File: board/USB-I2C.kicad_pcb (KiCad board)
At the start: 2 copper layers, 55 x 18 mm, 16 parts, among them J1 USB_OTG, J2 Conn_01x06, J3 Conn_01x06, U1 SPX3819, U2 ATSAMD11C14A-SS, X1 I2C-6P, X2 I2C, X3 SWD

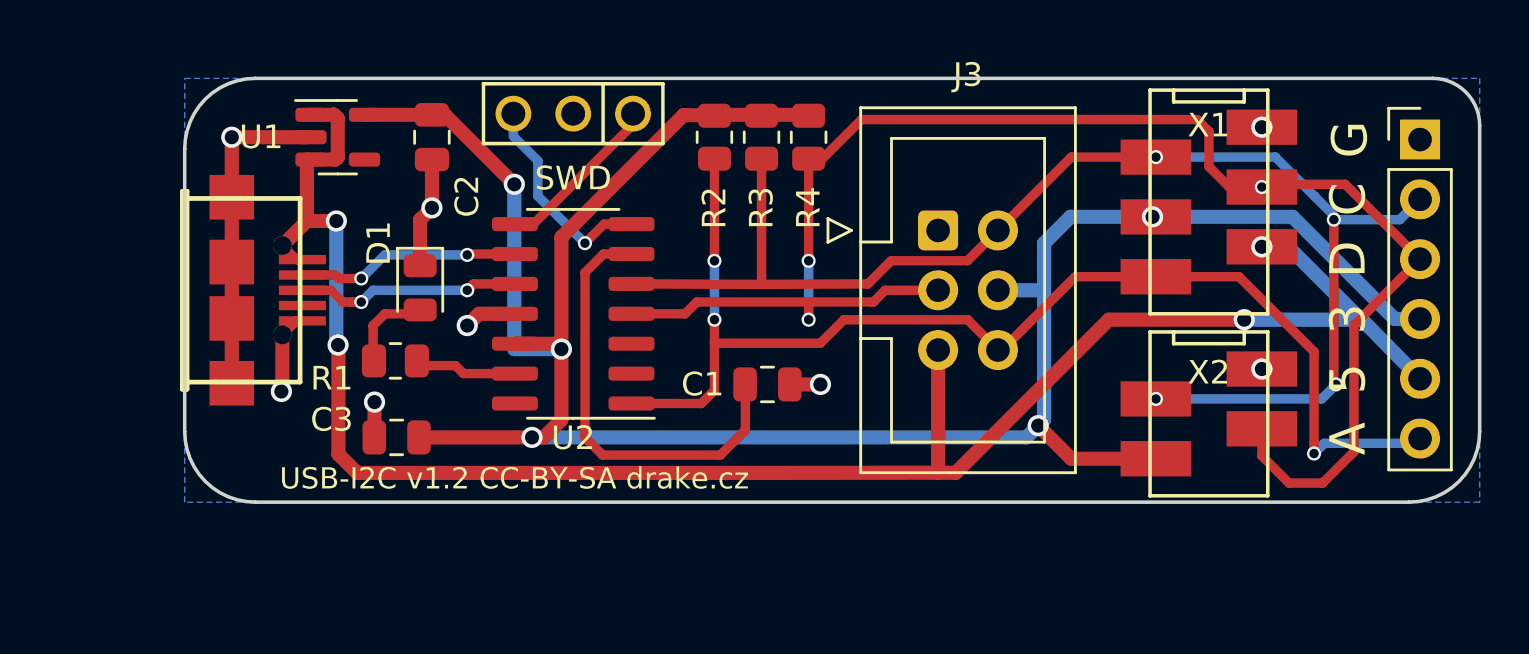
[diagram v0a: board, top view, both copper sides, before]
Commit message: WIP
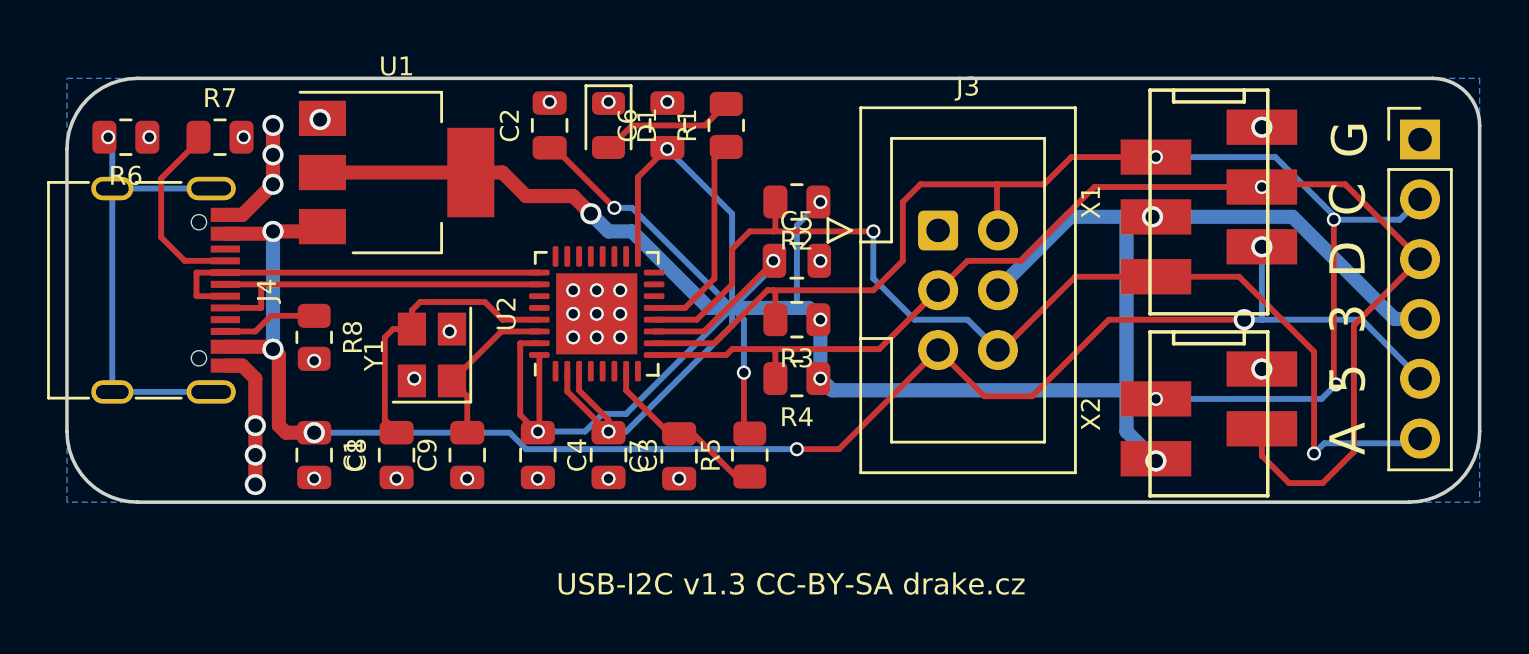
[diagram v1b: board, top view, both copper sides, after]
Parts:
- removed the C3 at (156.0, 114.2)
- removed the J1 at (149.0, 108.0)
- removed X3: SWD, Drake:SWD
- added C1: 10u, Capacitor_SMD:C_0805_2012Metric, F.Cu at (152.5, 115.0)
- added C4: 100n, Capacitor_SMD:C_0805_2012Metric, F.Cu at (162.0, 115.0)
- added C5: 100n, Capacitor_SMD:C_0805_2012Metric, F.Cu at (173.0, 106.8)
- added C6: 100n, Capacitor_SMD:C_0805_2012Metric, F.Cu at (167.5, 101.0)
- added C7: 1u, Capacitor_SMD:C_0805_2012Metric, F.Cu at (168.0, 115.0)
- added C8: 15p, Capacitor_SMD:C_0805_2012Metric, F.Cu at (156.0, 115.0)
- added C9: 15p, Capacitor_SMD:C_0805_2012Metric, F.Cu at (159.0, 115.0)
- added J4: USB_C_Receptacle, Connector_USB:USB_C_Receptacle_G-Switch_GT-USB-7010ASV, F.Cu at (145.0, 108.0)
- added R5: 10k, Resistor_SMD:R_0805_2012Metric, F.Cu at (171.0, 115.0)
- added R6: 1M, Resistor_SMD:R_0805_2012Metric, F.Cu at (144.5, 101.5)
- added R7: 5.11k 1%, Resistor_SMD:R_0805_2012Metric, F.Cu at (148.5, 101.5)
- added R8: 5.11k 1%, Resistor_SMD:R_0805_2012Metric, F.Cu at (152.5, 110.0)
- added Y1: 40MHz, Crystal:Crystal_SMD_3225-4Pin_3.2x2.5mm, F.Cu at (157.5, 110.8)
- C2: value 1u -> 10u
- U1: value SPX3819 -> LM1117MP-3.3; footprint Package_TO_SOT_SMD:SOT-23-5 -> Package_TO_SOT_SMD:SOT-223-3_TabPin2
- U2: value ATSAMD11C14A-SS -> ESP32-C3; footprint Package_SO:SOIC-14_3.9x8.7mm_P1.27mm -> Package_DFN_QFN:QFN-32-1EP_5x5mm_P0.5mm_EP3.45x3.45mm
- moved R1 17.2 mm to (170.0, 101.0), turned to 90 degrees
- moved D1 10.6 mm to (165.0, 101.0)
- moved R4 10.3 mm to (173.0, 111.8), turned to 180 degrees
- moved R3 7.89 mm to (173.0, 109.2), turned to 180 degrees
- moved C3 7.39 mm to (165.0, 115.0), turned to -90 degrees
- moved C2 5.02 mm to (162.5, 101.0), turned to 90 degrees
- moved R2 4.45 mm to (173.0, 104.2), turned to 180 degrees
- moved U1 2.92 mm to (156.0, 103.0)
- moved U2 1.00 mm to (164.5, 109.0), turned to 90 degrees
- renumbered C1 to C3, J2 to J1
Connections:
- C3 pad 1: Net-(C1-Pad1) -> +3V3
- U1 pad 1: +5V -> GND
- U1 pad 2: GND -> +3V3
- U2 pad 1: /ALERT -> unconnected-(U2-LNA_IN-Pad1)
- U2 pad 10: /USB_DP -> /SCL
- U2 pad 11: GND -> +3V3
- U2 pad 12: +3V3 -> /ALERT
- U2 pad 2: unconnected-(U2-Pad2) -> +3V3
- U2 pad 3: unconnected-(U2-Pad3) -> +3V3
- U2 pad 4: /SDA -> unconnected-(U2-XTAL_32K_P/ADC1_CH0-Pad4)
- U2 pad 5: /SCL -> unconnected-(U2-XTAL_32K_N/ADC1_CH1-Pad5)
- U2 pad 6: Net-(C1-Pad1) -> unconnected-(U2-GPIO2/ADC1_CH2-Pad6)
- U2 pad 7: /SWCLK -> Net-(U2-CHIP_EN)
- U2 pad 8: /SWDIO -> unconnected-(U2-GPIO3/ADC1_CH3-Pad8)
- U2 pad 9: /USB_DM -> /SDA
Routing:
- net +3V3: track 100.8 -> 149.0 mm, vias 5 -> 12
- net Net-(J4-SHIELD): track 0.00 -> 19.3 mm, vias 0 -> 1
- net Net-(C1-Pad1): track 18.8 -> 0.00 mm
- net GND: track 26.7 -> 11.1 mm, vias 8 -> 33
- net /SDA: track 66.5 -> 53.6 mm, vias 3 -> 1
- net Net-(U2-XTAL_N): track 0.00 -> 12.2 mm
- net +5V: track 81.5 -> 71.6 mm, vias 4 -> 6
- net /SWCLK: track 9.41 -> 0.00 mm, vias 1 -> 0
- net Net-(J4-CC1): track 0.00 -> 8.05 mm
- net Net-(U2-CHIP_EN): track 0.00 -> 7.58 mm
- net /USB_DM: track 9.52 -> 16.8 mm, vias 2 -> 0
- net /SWDIO: track 7.23 -> 0.00 mm
- net Net-(U2-XTAL_P): track 0.00 -> 7.05 mm
- net /USB_DP: track 9.55 -> 15.9 mm, vias 2 -> 0
- net /ALERT: track 52.4 -> 47.4 mm, vias 3 -> 2
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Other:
- board size 55 x 18 mm -> 60 x 18 mm
- rule pad_to_mask_clearance: 0.2 -> 0.05
- rule solder_mask_min_width: 0.25 -> 0.254
- board text added: "USB-I2C v1.3 CC-BY-SA drake.cz"
- board text removed: "SWD"
- board text removed: "USB-I2C v1.2 CC-BY-SA drake.cz"

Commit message: WIP
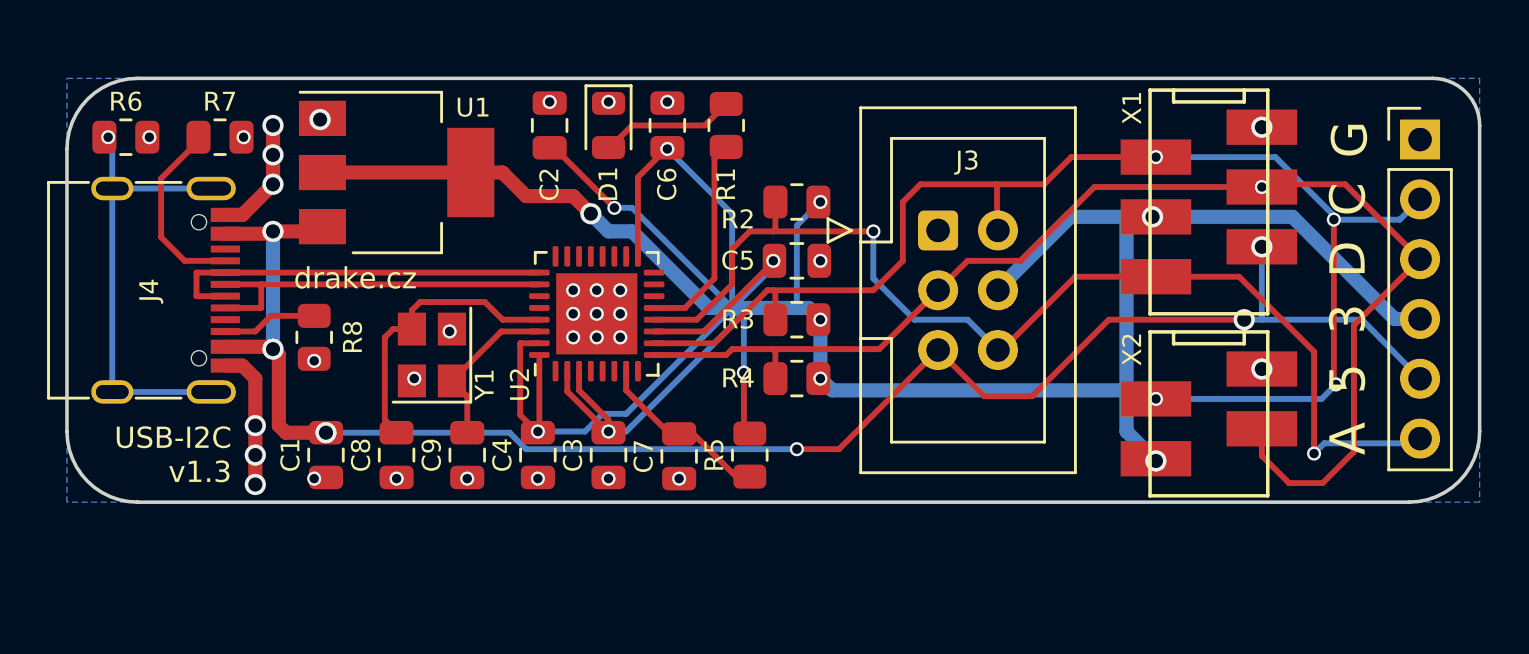
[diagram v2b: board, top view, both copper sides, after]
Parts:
- moved C1 0.50 mm to (153.0, 115.0)
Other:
- board text added: "USB-I2C v1.3"
- board text added: "drake.cz"
- board text removed: "USB-I2C v1.3 CC-BY-SA drake.cz"
